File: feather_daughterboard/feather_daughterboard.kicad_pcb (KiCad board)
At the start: 2 copper layers, 79.7 x 11 mm, 20 parts, among them J1 61900619521

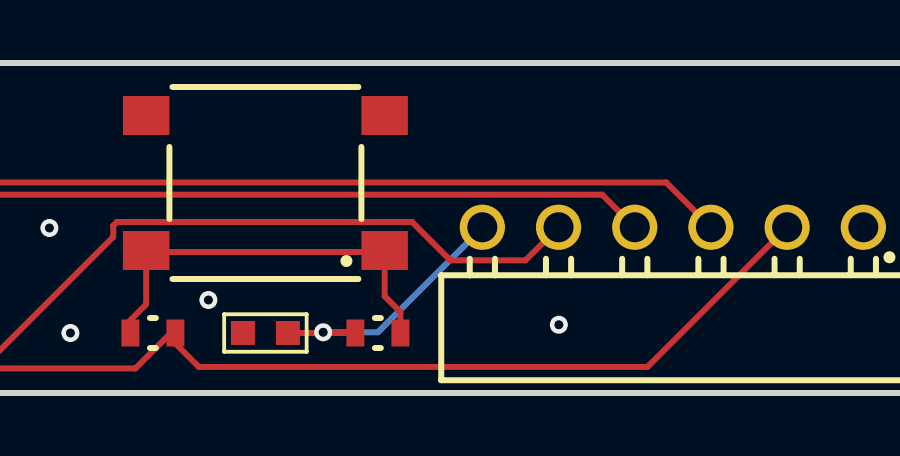
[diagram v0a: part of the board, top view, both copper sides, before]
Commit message: finished the mainboard, added bom files
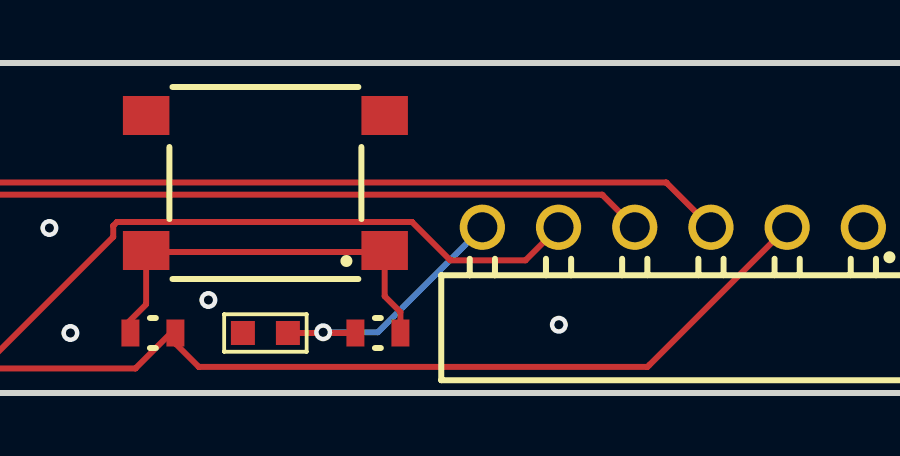
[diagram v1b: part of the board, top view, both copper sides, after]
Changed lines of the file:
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@@
 	(generator_version "8.0")
 	(general
-		(thickness 1.6)
+		(thickness 1.579)
 		(legacy_teardrops no)
 	)
@@
 	)
 	(setup
+		(stackup
+			(layer "F.SilkS"
+				(type "Top Silk Screen")
+				(color "White")
+				(material "Peters SD2692")
+			)
+			(layer "F.Paste"
+				(type "Top Solder Paste")
+			)
+			(layer "F.Mask"
+				(type "Top Solder Mask")
+				(color "Green")
+				(thickness 0.025)
+				(material "Elpemer AS 2467 SM-DG")
+				(epsilon_r 3.7)
+				(loss_tangent 0)
+			)
+			(layer "F.Cu"
+				(type "copper")
+				(thickness 0.035)
+			)
+			(layer "dielectric 1"
+				(type "core")
+				(color "FR4 natural")
+				(thickness 1.459)
+				(material "FR4")
+				(epsilon_r 4.5)
+				(loss_tangent 0.02)
+			)
+			(layer "B.Cu"
+				(type "copper")
+				(thickness 0.035)
+			)
+			(layer "B.Mask"
+				(type "Bottom Solder Mask")
+				(color "Green")
+				(thickness 0.025)
+				(material "Elpemer AS 2467 SM-DG")
+				(epsilon_r 3.7)
+				(loss_tangent 0)
+			)
+			(layer "B.Paste"
+				(type "Bottom Solder Paste")
+			)
+			(layer "B.SilkS"
+				(type "Bottom Silk Screen")
+				(color "White")
+				(material "Peters SD2692")
+			)
+			(copper_finish "ENIG")
+			(dielectric_constraints no)
+		)
 		(pad_to_mask_clearance 0)
 		(allow_soldermask_bridges_in_footprints no)
@@
 		(width 0.2)
 		(layer "F.Cu")
-		(net 3)
-	)
-	(segment
-		(start 164.64055 85.5533)
-		(end 164.66555 85.5783)
-		(width 0.2)
-		(layer "F.Cu")
